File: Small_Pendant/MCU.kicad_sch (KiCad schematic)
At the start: 45 parts, among them J1 USB_C_Receptacle_USB2.0_16P, J2 Interboard, J3 Interboard, J4 Interboard, SW1 SW_Push, SW2 SW_Push, SW3 SW_Push, U1 ESP32-C3-MINI-1, U2 AP2112K-3.3, U3 BNO055, U4 SN74LVC1T45DCK

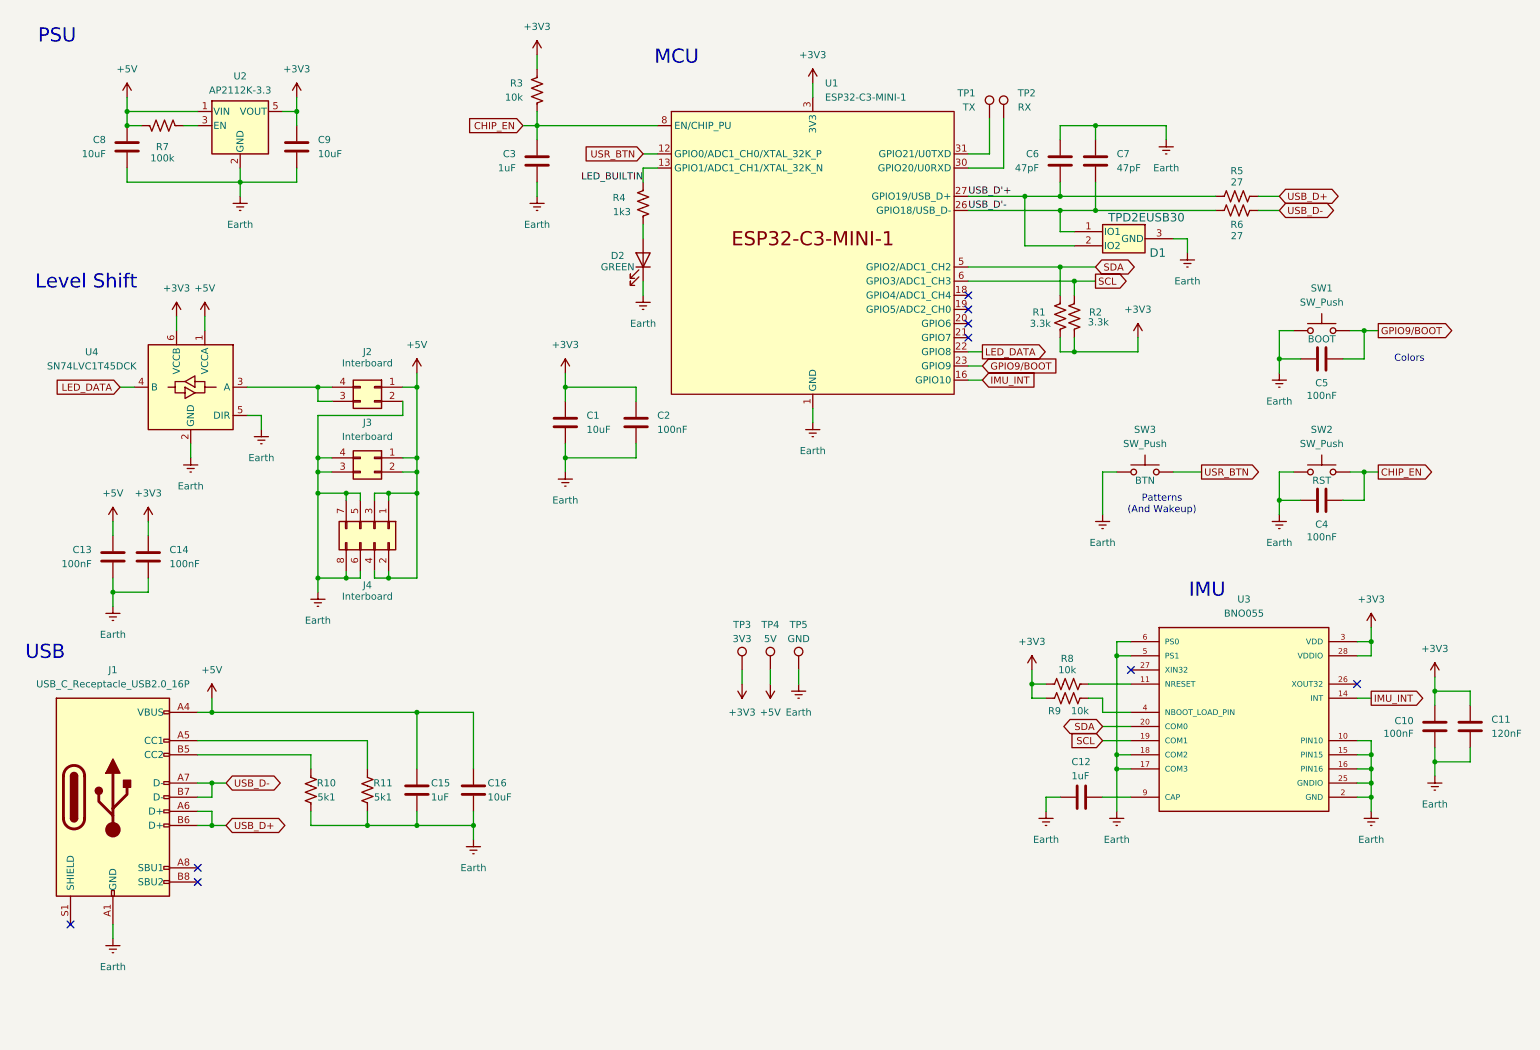
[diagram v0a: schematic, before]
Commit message: [HW] Schematic and Layout/Routing Clean Up
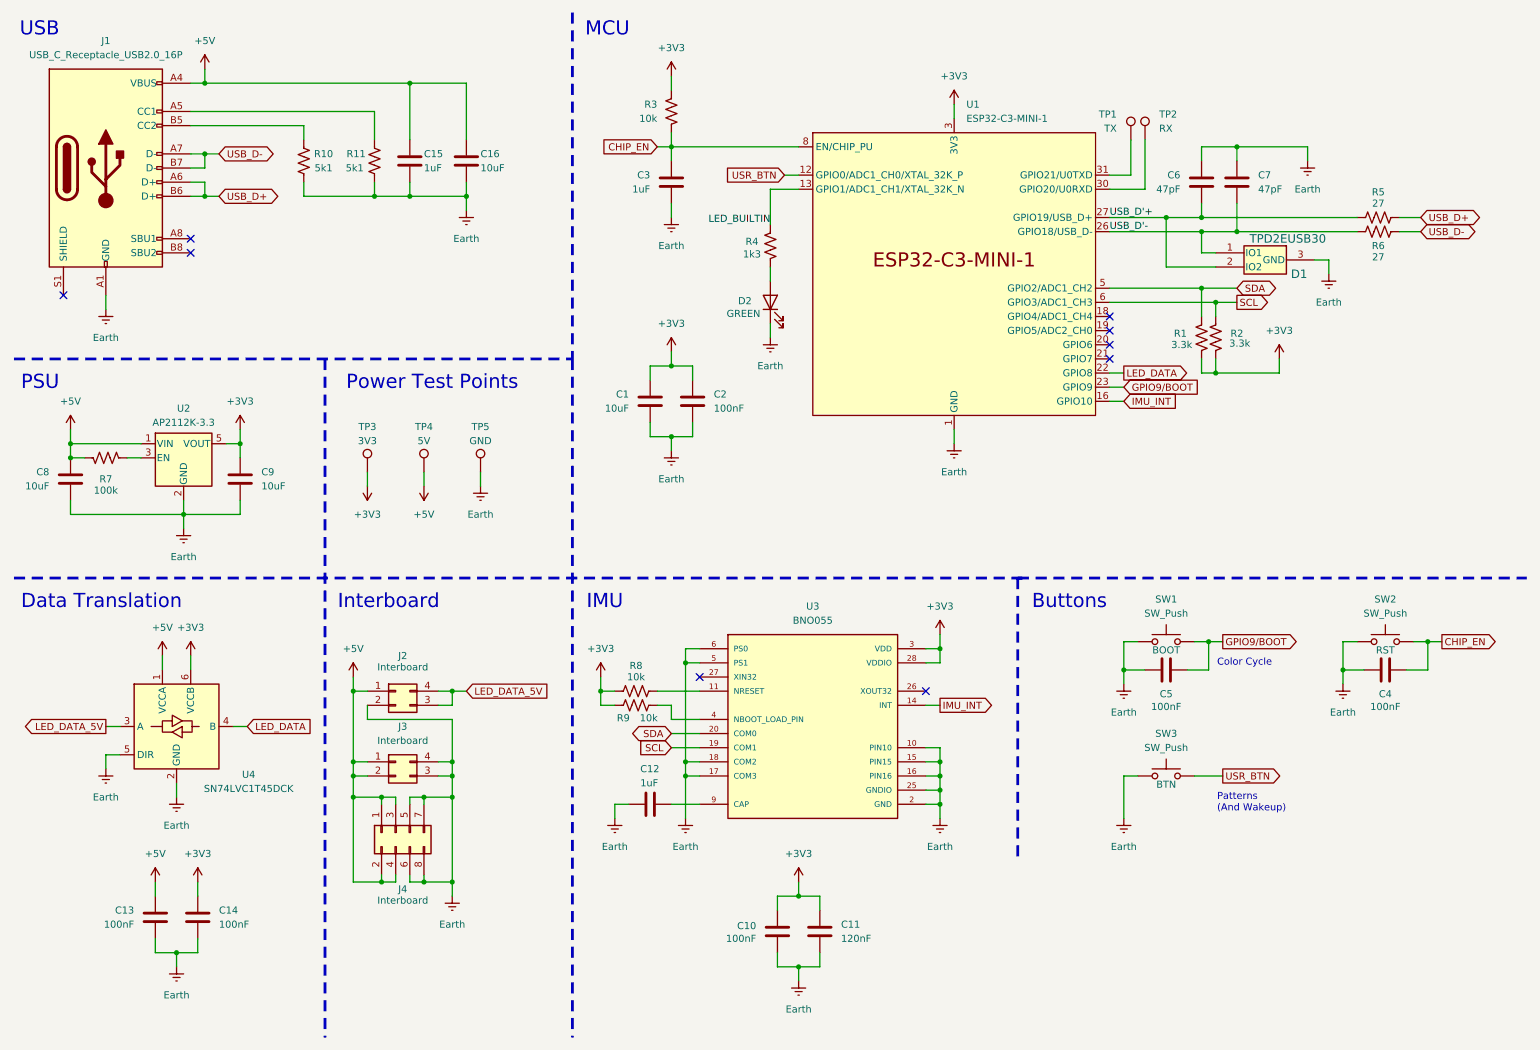
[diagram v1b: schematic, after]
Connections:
- net LED_BUILTIN: now also R4.2; no longer R4.1
- net at D2.2 (A): now also R4.1; no longer R4.2
- net LED_DATA_5V: now reaches J2.3 (Pin_3), J2.4 (Pin_4), U4.3 (A)
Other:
- note added: "Buttons"
- note added: "Color Cycle"
- note added: "Data Translation"
- note added: "Interboard"
- note added: "Power Test Points"
- note removed: "Colors"
- note removed: "Level Shift"
- moved on the sheet: C1, C10, C11, C12, C13, C14, C15, C16, C2, C3, C4, C5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

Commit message: [Docs] Lots added to the Readme, BOM, schematics,...
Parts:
- J1: LCSC Part C3020560 -> C2988366
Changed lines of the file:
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@@
 			)
 		)
-		(property "LCSC Part" "C3020560"
+		(property "LCSC Part" "C2988366"
 			(at 29.21 40.64 0)
 			(effects

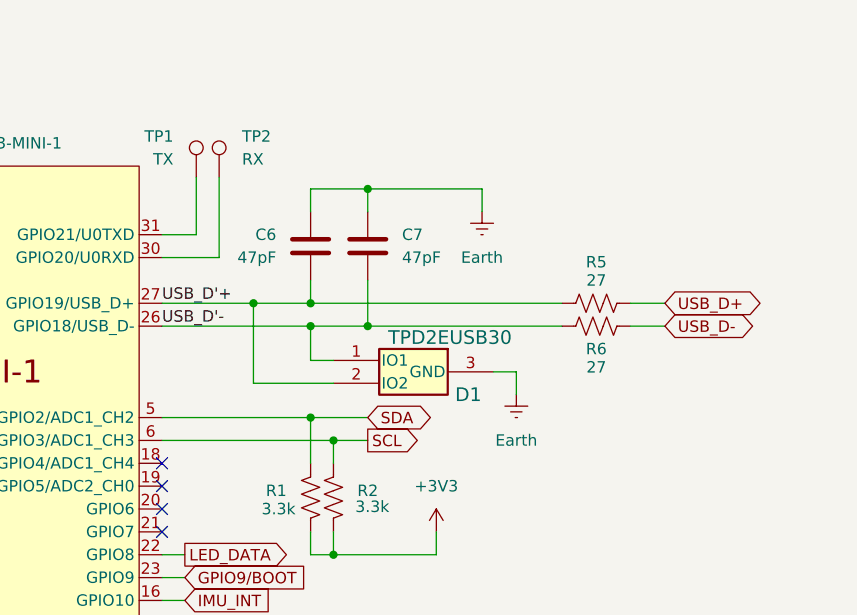
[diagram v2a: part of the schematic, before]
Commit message: [HW] Clean up ESD Diode
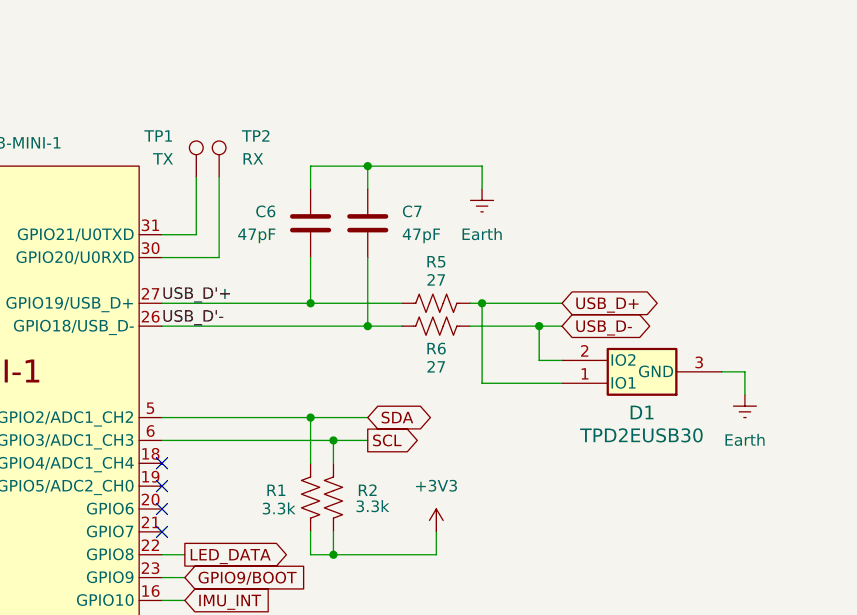
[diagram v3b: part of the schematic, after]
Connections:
- net USB_D'+: no longer D1.2 (IO2)
- net USB_D'-: no longer D1.1 (IO1)
- net USB_D+: now also D1.1 (IO1)
- net USB_D-: now also D1.2 (IO2)
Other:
- moved on the sheet: C6, C7, D1, R5, R6
